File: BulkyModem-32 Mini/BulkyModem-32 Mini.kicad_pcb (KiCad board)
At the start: 2 copper layers, 38.7 x 73 mm, 26 parts, among them J1 SD_CARD, J2 DCE, U3 MAX232, U6 74HCT32

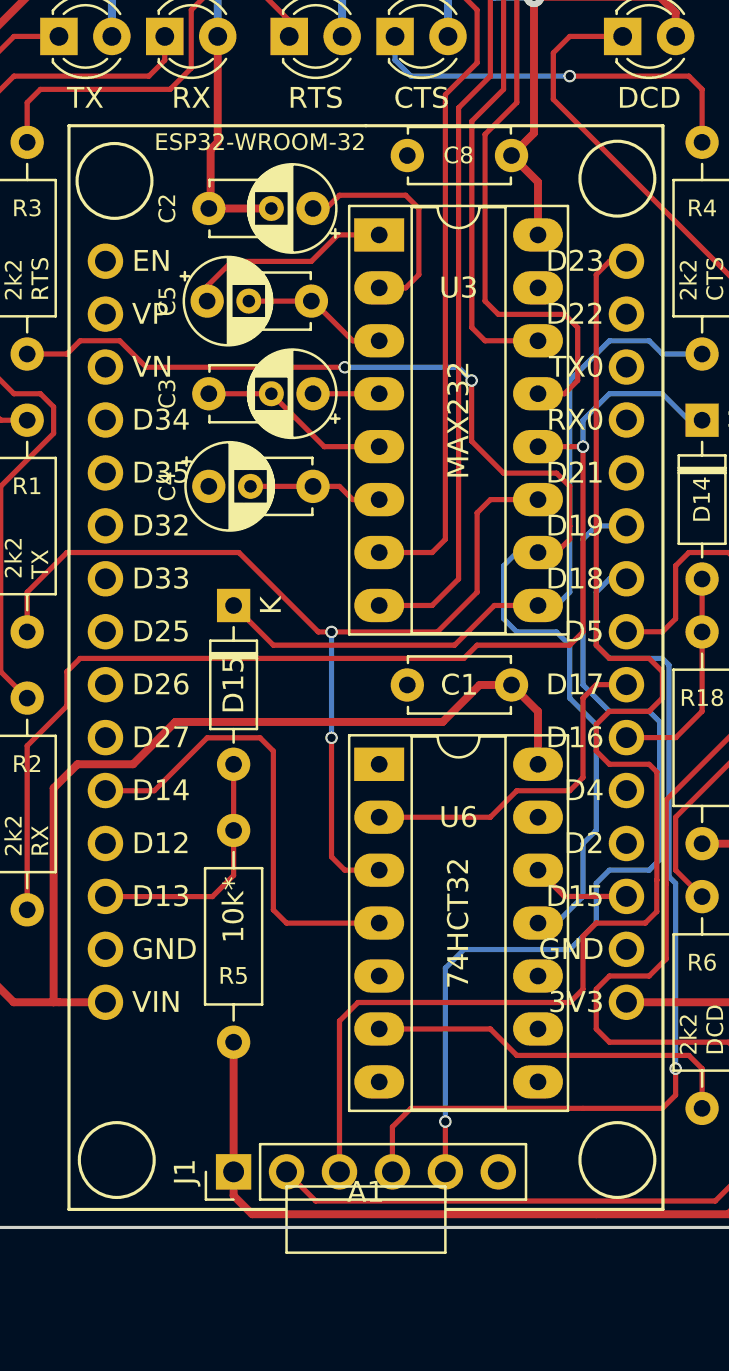
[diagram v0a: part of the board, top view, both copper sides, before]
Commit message: ESP32 Mini cleanup
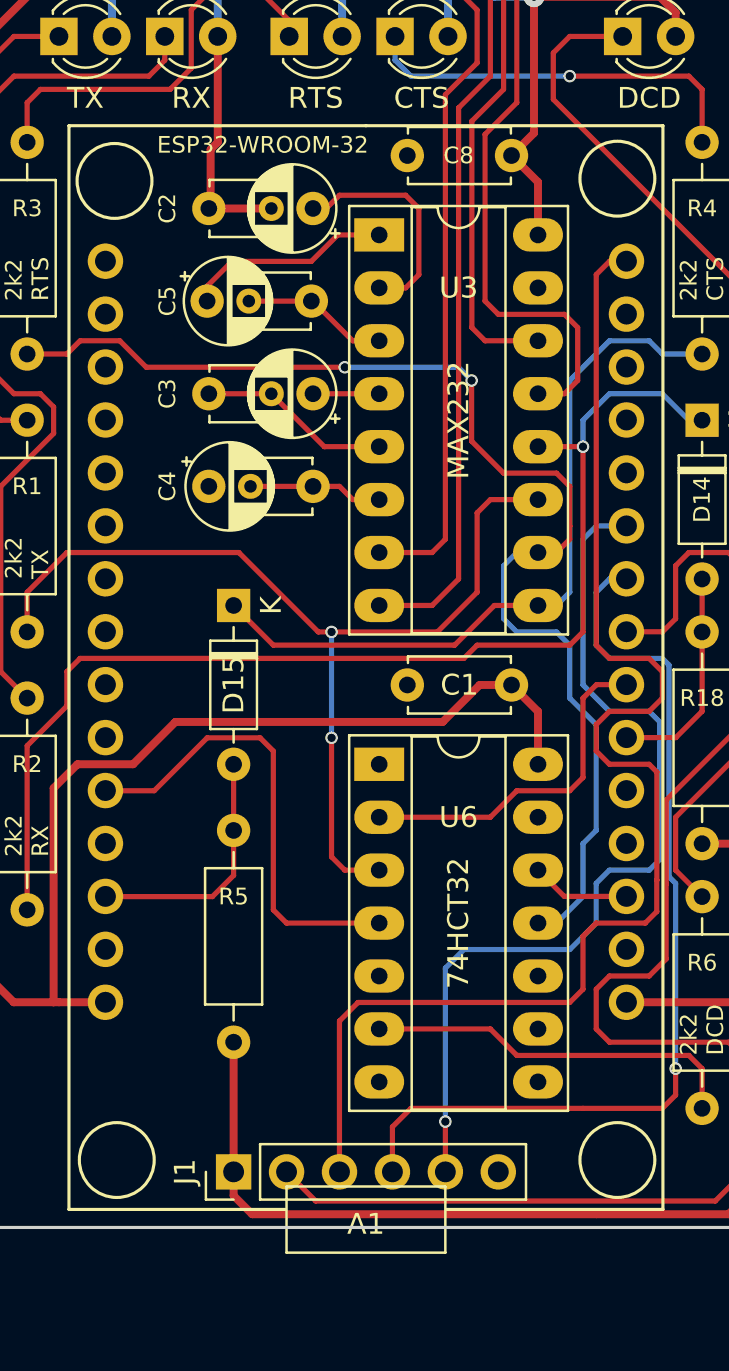
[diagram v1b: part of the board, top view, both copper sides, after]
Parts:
- A1: footprint esp32_dev_board:ESP32-WROOM-32D_30 -> esp32_dev_board:ESP32-WROOM-32D_30_Alternate
